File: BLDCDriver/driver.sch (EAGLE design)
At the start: 72 parts, among them Q1 NJM7800S, U1 QFN50P400X400X100-25NDRV8300D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, U2 AS5048A-HTSP-500, U4 SOP80P620X125-8N

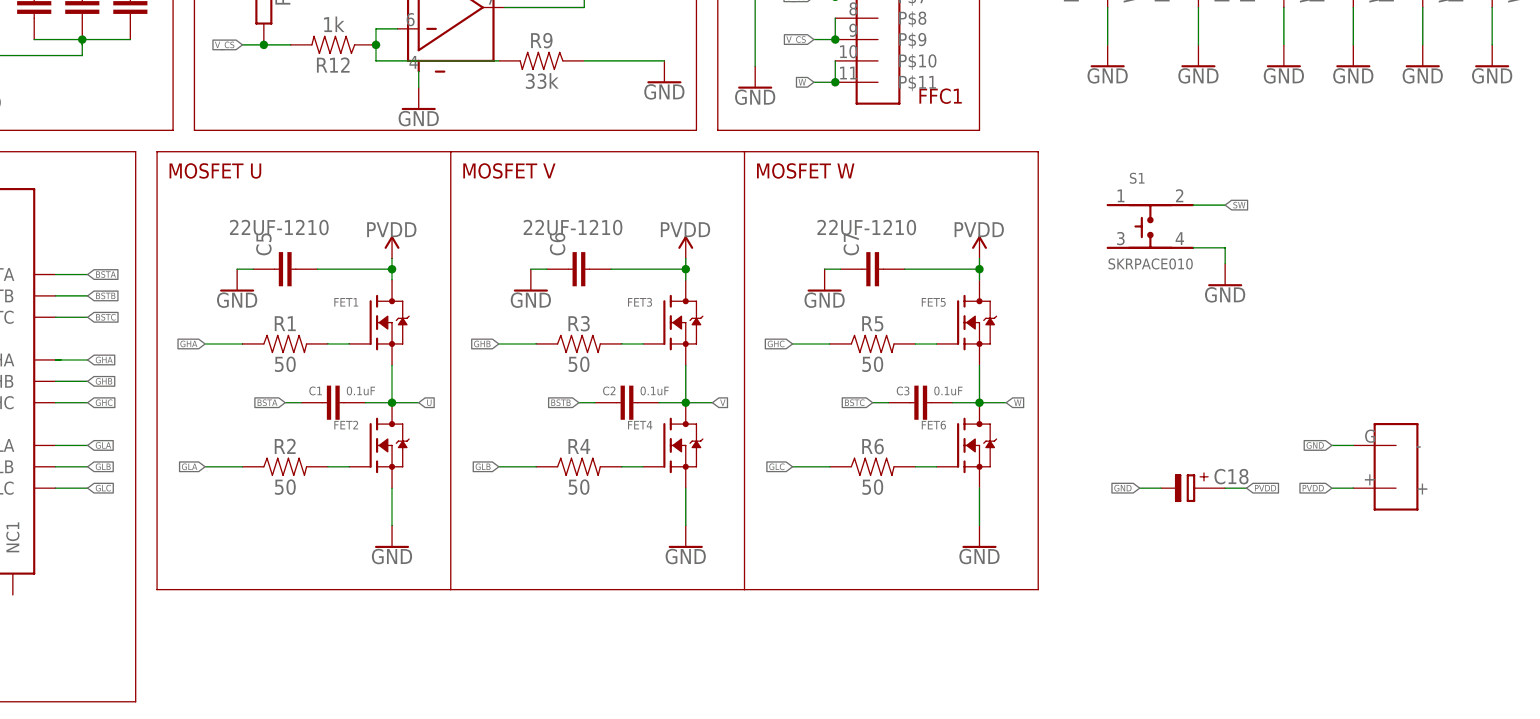
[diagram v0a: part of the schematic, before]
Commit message: 救いはないんですか〜？
# ==== Emojis ====
# ✨ :sparkles: Add new feature
# ✅  :white_check_mark: Update existing feature (not bug)
# ⚠️  :warning: Fix bug/error
# 🔥  :fire: Remove files or features
# ✏️ :pencil2: Fix typos
# 📝  :memo: Update documentation
# ♻️  :recycle: Dependencies update
# 🐧  :penguin: Improved the Linux
# 🍎  :apple: Improved the macOS
# 🔖 :bookmark: Add new library
# 🎉  :tada: Initial commit

# ==== Format ====
# :emoji: Subject
#
# Commit body...

# ==== Messages ====
# 新規(ファイル)機能追加: Add
# 機能修正、既存機能追加（バグではない): Update
# リファクタリング: Clean
# ファイル名変更:
# 削除など: Remove
# バグ修正: Fix
# バージョンアップ: Upgrade
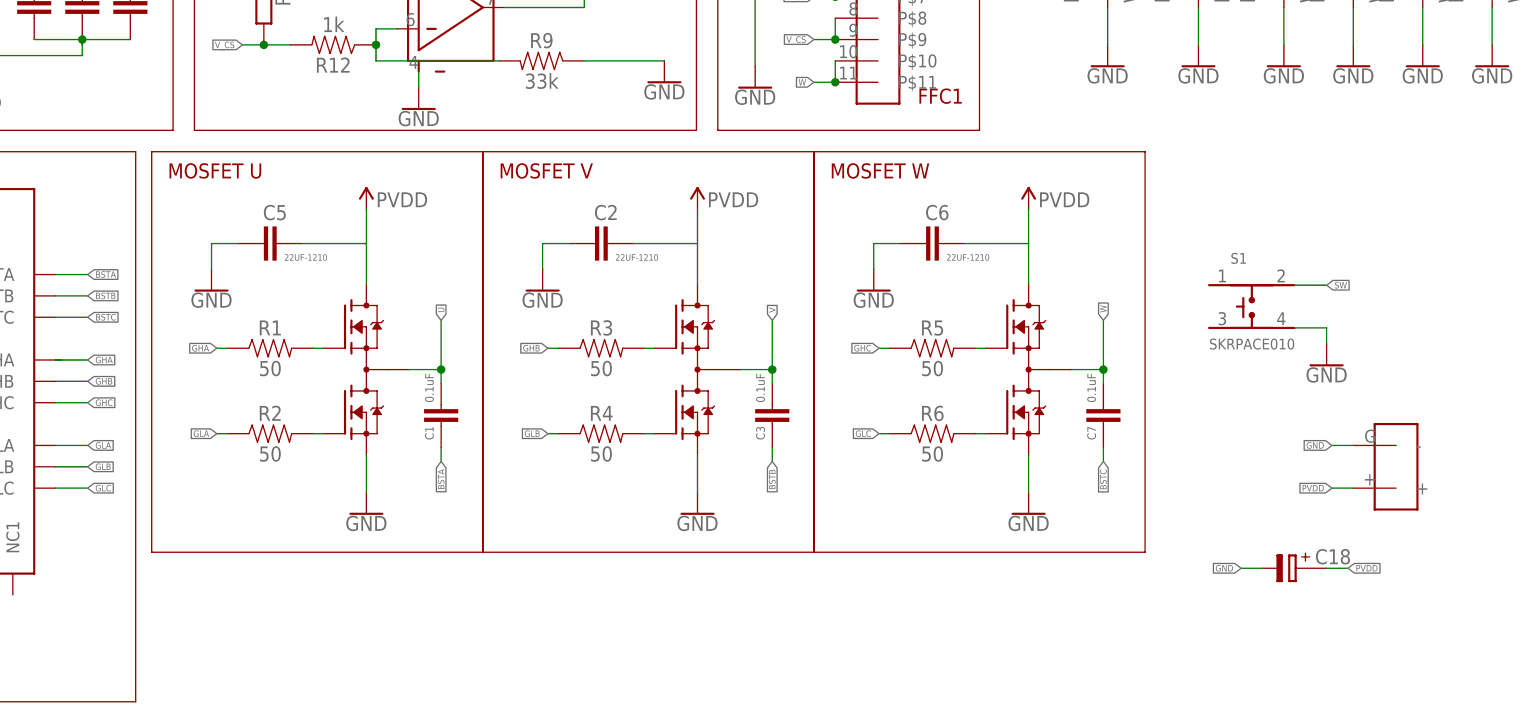
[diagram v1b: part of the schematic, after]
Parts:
- removed FET1, FET2, FET3, FET4, FET5, FET6: TPH11006NL, TPH11006NL:TPH11006NL
- added Q2, Q3, Q4: SIZ240DT-T1-GE3, SIZ240DT-T1-GE3:SIZ240DT-T1-GE3
- C2: value 0.1uF -> 22UF-1210; device SparkFun-Capacitors:0.1UF-0603-25V-5% -> SparkFun-Capacitors:22UF-1210-16V-20%
- C7: value 22UF-1210 -> 0.1uF; device SparkFun-Capacitors:22UF-1210-16V-20% -> SparkFun-Capacitors:0.1UF-0603-25V-5%
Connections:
- net BSTB: now also C3.1; no longer C2.1
- net BSTC: now also C7.1; no longer C3.1
- net GND: now also C2.1, Q2.S2, Q3.S2, Q4.S2; no longer C7.1, FET2.S, FET4.S, FET6.S
- net N$1: now also Q3.G1; no longer FET3.G
- net N$2: now also Q2.G1; no longer FET1.G
- net N$4: now also Q2.G2; no longer FET2.G
- net N$5: now also Q3.G2; no longer FET4.G
- net N$6: now also Q4.G1; no longer FET5.G
- net N$7: now also Q4.G2; no longer FET6.G
- net PVDD: now also C2.2, Q2.D1, Q3.D1, Q4.D1; no longer C7.2, FET1.D, FET3.D, FET5.D
- net U: now also Q2.S1/D2; no longer FET1.S, FET2.D
- net V: now also C3.2, Q3.S1/D2; no longer C2.2, FET3.S, FET4.D
- net W: now also C7.2, Q4.S1/D2; no longer C3.2, FET5.S, FET6.D
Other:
- moved on the sheet: C1, C18, C2, C3, C5, C6, C7, R1, R2, R3, R4, R5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
